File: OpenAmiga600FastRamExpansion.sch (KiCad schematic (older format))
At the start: 27 parts, among them J1 MC68000_PLCC68, P1 JTAG_CONNECTOR, P98 SCREW_HOLE, P99 OSHW_LOGO, U1 74LS157, U2 74LS157, U3 HYB5118160BSJ, U4 HYB5118160BSJ, U5 ATF1502AS-10JU44

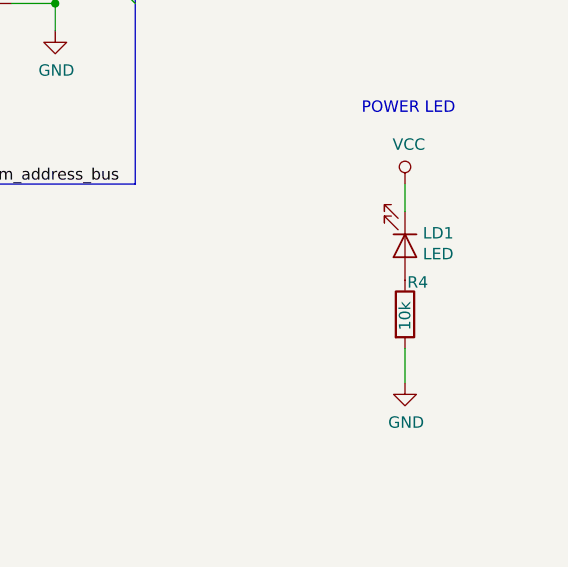
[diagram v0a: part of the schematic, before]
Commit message: Fix #1
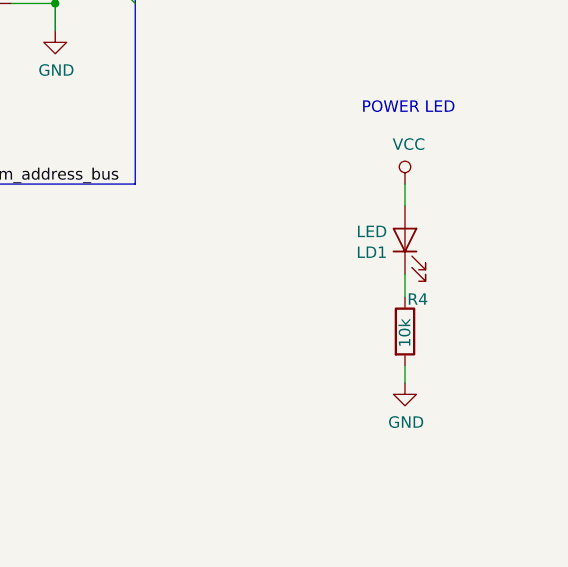
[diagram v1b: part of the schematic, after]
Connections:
- wire segments 351 -> 352
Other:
- moved on the sheet: LD1, R4
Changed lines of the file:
@@
 $EndComp
 Wire Wire Line
-	15260 8500 15260 8620
-Wire Wire Line
-	15260 9220 15260 9370
+	15260 8500 15260 8595
 $Comp
 L Device:LED LD1
 U 1 1 5CBAB2B0
-P 15260 8770
-F 0 "LD1" V 15205 8848 50  0000 L CNN
-F 1 "LED" V 15296 8848 50  0000 L CNN
-F 2 "OpenAmiga600FastRamExpansion:LED_0805_HandSoldering_ModSilkS" H 15260 8770 50  0001 C CNN
-F 3 "~" H 15260 8770 50  0001 C CNN
-	1    15260 8770
-	0    1    1    0
+P 15260 8745
+F 0 "LD1" V 15205 8823 50  0000 L CNN
+F 1 "LED" V 15296 8823 50  0000 L CNN
+F 2 "OpenAmiga600FastRamExpansion:LED_0805_HandSoldering_ModSilkS" H 15260 8745 50  0001 C CNN
+F 3 "~" H 15260 8745 50  0001 C CNN
+	1    15260 8745
+	0    -1   -1   0
 $EndComp
 $Comp
 L Device:R R4
 U 1 1 5CBCAA9F
-P 15260 9070
-F 0 "R4" H 15270 9210 50  0000 L CNN
-F 1 "10k" V 15260 9000 50  0000 L CNN
-F 2 "Resistor_SMD:R_0805_2012Metric_Pad1.15x1.40mm_HandSolder" V 15190 9070 50  0001 C CNN
-F 3 "~" H 15260 9070 50  0001 C CNN
-	1    15260 9070
+P 15260 9145
+F 0 "R4" H 15270 9285 50  0000 L CNN
+F 1 "10k" V 15260 9075 50  0000 L CNN
+F 2 "Resistor_SMD:R_0805_2012Metric_Pad1.15x1.40mm_HandSolder" V 15190 9145 50  0001 C CNN
+F 3 "~" H 15260 9145 50  0001 C CNN
+	1    15260 9145
 	1    0    0    -1
 $EndComp
@@
 Wire Wire Line
 	11330 10530 11330 10620
+Wire Wire Line
+	15260 9295 15260 9370
+Wire Wire Line
+	15260 8895 15260 8995
 Wire Bus Line
 	11610 4190 11610 8500
